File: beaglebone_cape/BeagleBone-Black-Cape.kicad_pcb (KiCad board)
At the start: 2 copper layers, 54.6 x 86.4 mm, 49 parts, among them J1 MC000052, J10 MOLEX_2031, J11 MOLEX_2021, J12 EBV-02-D, J2 MOLEX_2051, J3 MOLEX_2031, J4 MOLEX_2021, J5 MOLEX_2041, J6 MOLEX_2031, J7 MOLEX_2041, J8 MOLEX_2031, J9 MOLEX_2041, P1 BeagleBone_Black_Header, P2 BeagleBone_Black_Header, Q1 IRLB8721PBF, Q2 IRFML8244, U1 DIGIPOT_50K, U2 U_IC-HKB, U3 X_STEPPER, U4 Y_STEPPER, U5 Z_STEPPER

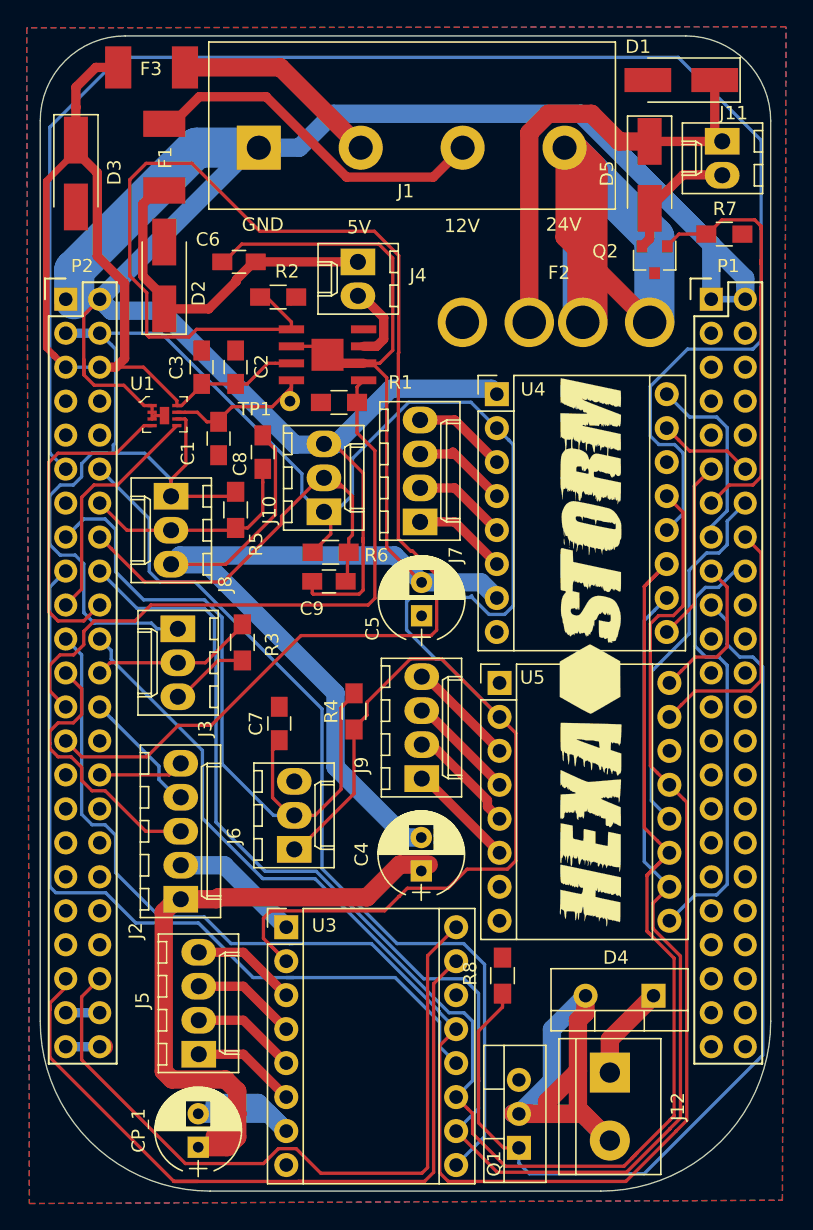
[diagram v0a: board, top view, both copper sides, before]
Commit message: finished layout of all PCBs
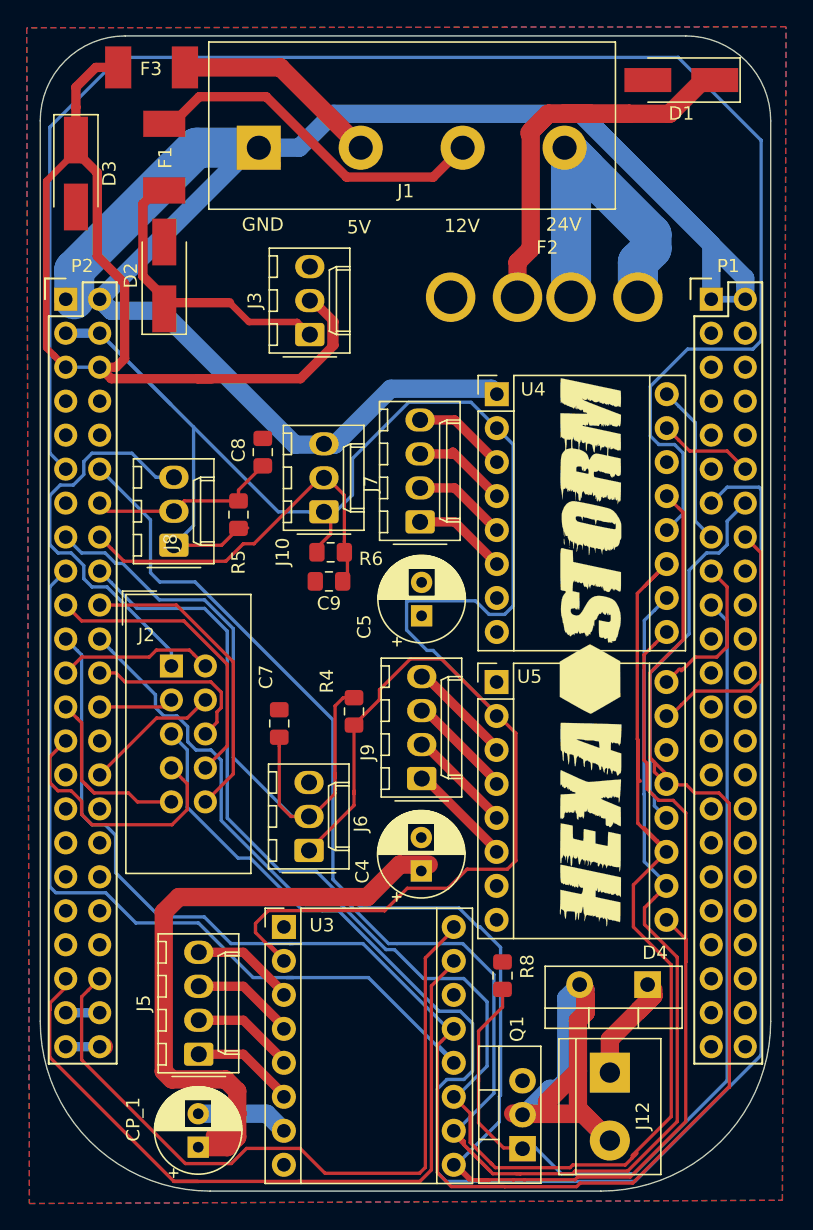
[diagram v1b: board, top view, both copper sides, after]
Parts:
- removed C1: 47nF, Capacitors_SMD:C_0805_HandSoldering
- removed C2, C6: 1uF, Capacitors_SMD:C_0805_HandSoldering
- removed C3: 0.1uF, Capacitors_SMD:C_0805_HandSoldering
- removed D5: 50V_1A, Diodes_SMD:D_SMA_Handsoldering
- removed J11, J4: MOLEX_2021, Connectors_Molex:Molex_KK-6410-02_02x2.54mm_Straight
- removed Q2: IRFML8244, TO_SOT_Packages_SMD:SOT-23
- removed R1, R2, R7: 10K, Resistors_SMD:R_0805_HandSoldering
- removed R3: 340K, Resistors_SMD:R_0805_HandSoldering
- removed TP1: TestPoint, Measurement_Points:Measurement_Point_Round-TH_Small
- removed U1: DIGIPOT_50K, Socket_BeagleBone_Black:TDFN-8-1EP
- removed U2: U_IC-HKB, Socket_BeagleBone_Black:ICHKB
- C4, C5, CP_1: footprint Capacitors_THT:CP_Radial_D6.3mm_P2.50mm -> Capacitor_THT:CP_Radial_D6.3mm_P2.50mm
- C7, C8, C9: footprint Capacitors_SMD:C_0805_HandSoldering -> Capacitor_SMD:C_0805_2012Metric_Pad1.15x1.40mm_HandSolder
- D1, D2, D3: footprint Diodes_SMD:D_SMA_Handsoldering -> Diode_SMD:D_SMA_Handsoldering
- D4: footprint TO_SOT_Packages_THT:TO-220-2_Vertical -> Package_TO_SOT_THT:TO-220-2_Vertical
- J10, J3, J6, J8: footprint Connectors_Molex:Molex_KK-6410-03_03x2.54mm_Straight -> Connector_Molex:Molex_KK-254_AE-6410-03A_1x03_P2.54mm_Vertical
- J12: footprint Connectors_Terminal_Blocks:TerminalBlock_bornier-2_P5.08mm -> TerminalBlock:TerminalBlock_bornier-2_P5.08mm
- J2: value MOLEX_2051 -> 10pinIDC; footprint Connectors_Molex:Molex_KK-6410-05_05x2.54mm_Straight -> Connector_IDC:IDC-Header_2x05_P2.54mm_Vertical
- J5, J7, J9: footprint Connectors_Molex:Molex_KK-6410-04_04x2.54mm_Straight -> Connector_Molex:Molex_KK-254_AE-6410-04A_1x04_P2.54mm_Vertical
- Q1: footprint TO_SOT_Packages_THT:TO-220-3_Vertical -> Package_TO_SOT_THT:TO-220-3_Vertical
- R4, R5, R6, R8: footprint Resistors_SMD:R_0805_HandSoldering -> Resistor_SMD:R_0805_2012Metric_Pad1.15x1.40mm_HandSolder
- moved J3 24.1 mm to (134.6, 65.0), turned to 90 degrees
- moved J2 17.5 mm to (124.3, 89.8), turned to 0 degrees
- moved J8 3.66 mm to (124.5, 80.8), turned to 90 degrees
- moved F2 2.07 mm to (152.1, 62.2)
- moved J6 1.11 mm to (134.6, 103.6)
- moved D4 0.94 mm to (159.9, 113.6)
- moved R5 0.42 mm to (129.3, 78.5), turned to 90 degrees
- moved Q1 0.28 mm to (150.5, 125.9)
- moved U5 0.23 mm to (148.6, 91.0)
- moved U3 0.18 mm to (132.7, 109.3)
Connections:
- J2 pad 1: +24V -> GND
- J2 pad 2: GND -> POLY_EN
- J2 pad 3: POLY_EN -> POLY_READY
- J2 pad 4: POLY_READY -> POLY_PWM
- J2 pad 5: POLY_PWM -> FAN_PWM
- J3 pad 1: +3V3 -> +12V
- J3 pad 2: PH_DIODE -> +5V
- P1 pad 11: Y_ENABLE -> Net-(P1-Pad11)
- P1 pad 18: Z_ENABLE -> Net-(P1-Pad18)
- P2 pad 12: X_ENABLE -> ENABLE
- U3 pad 1: X_ENABLE -> ENABLE
- U4 pad 1: Y_ENABLE -> ENABLE
- U5 pad 1: Z_ENABLE -> ENABLE
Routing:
- net GND: track 351.6 -> 205.6 mm
- net ENABLE: track 0.00 -> 137.4 mm
- net IC_HB_PWM2: track 111.6 -> 19.8 mm
- net FAN_PWM: track 33.0 -> 122.0 mm
- net X_ENABLE: track 69.3 -> 0.00 mm
- net IC_HB_PWM1: track 47.6 -> 14.1 mm
- net Z_ENABLE: track 33.0 -> 0.00 mm
- net +3V3: track 201.5 -> 169.8 mm
- net Net-(F2-Pad1): track 58.9 -> 29.7 mm
- net +5V: track 63.8 -> 85.7 mm
- net Y_ENABLE: track 13.6 -> 0.00 mm
- net POT_W: track 12.1 -> 0.00 mm
- net Net-(D5-Pad2): track 9.44 -> 0.00 mm
- net POLY_EN: track 20.7 -> 11.6 mm
- net SPIO_DI: track 122.9 -> 129.8 mm
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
